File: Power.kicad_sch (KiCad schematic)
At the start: 42 parts, among them J1 1769, U11 XC6206P302MR_C5148691, U6 EA3036C, U7 MT3608, U9 BQ24074RGTR

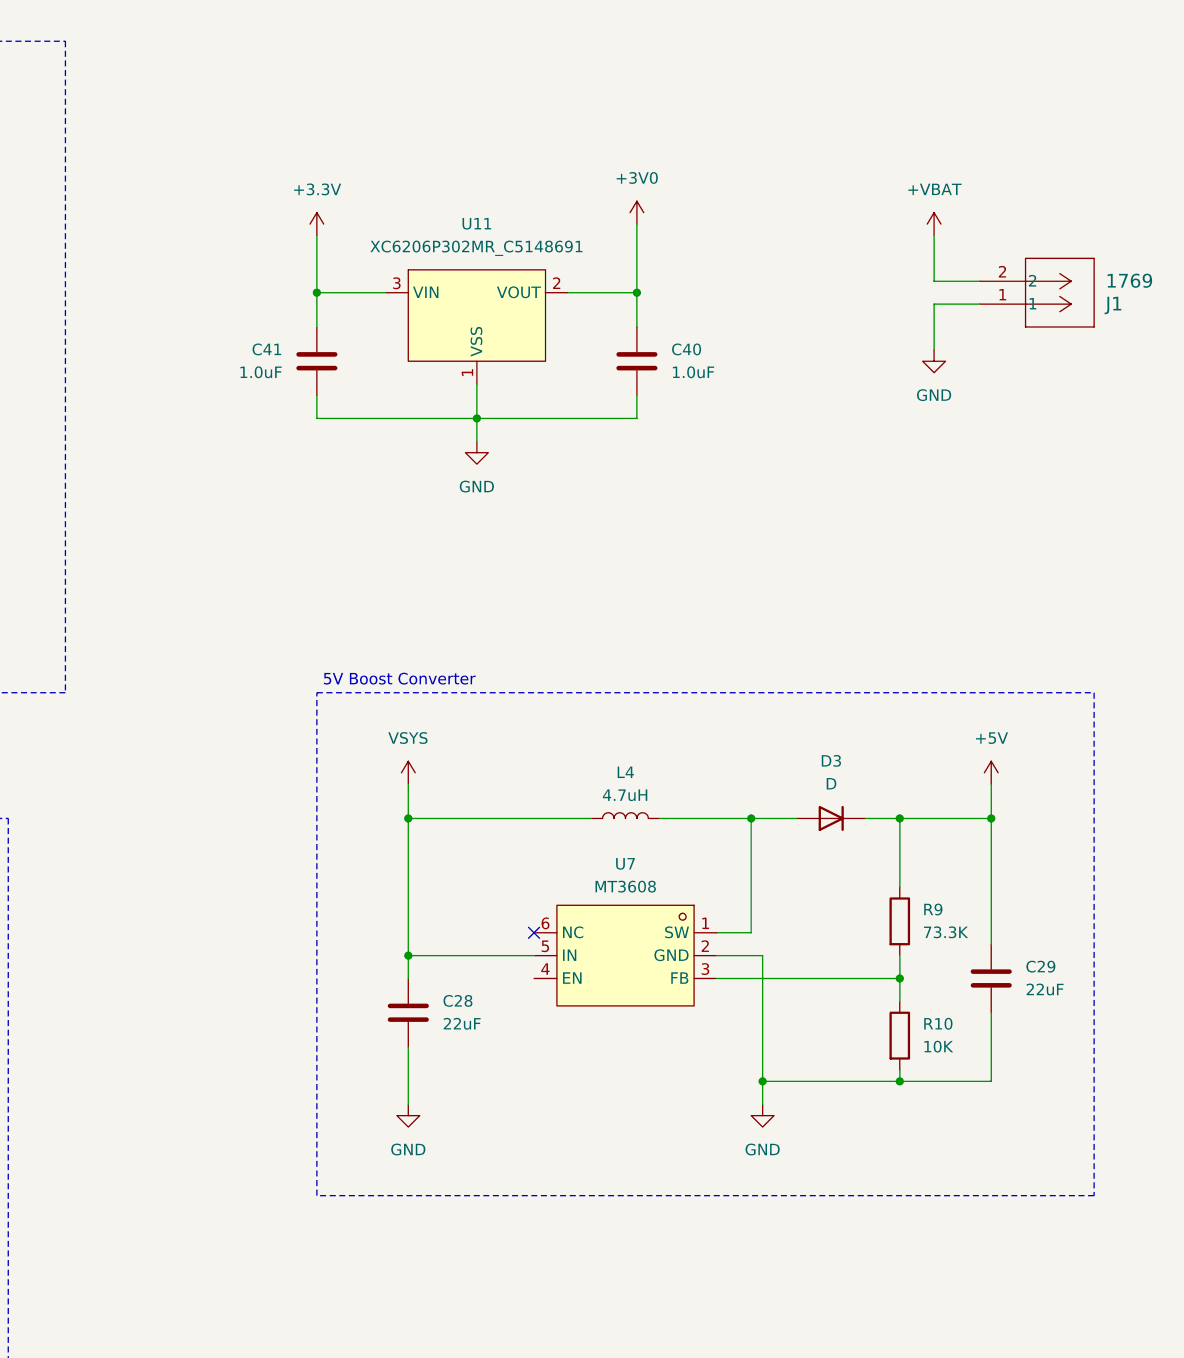
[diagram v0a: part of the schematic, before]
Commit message: power changes for v3s, cleanup
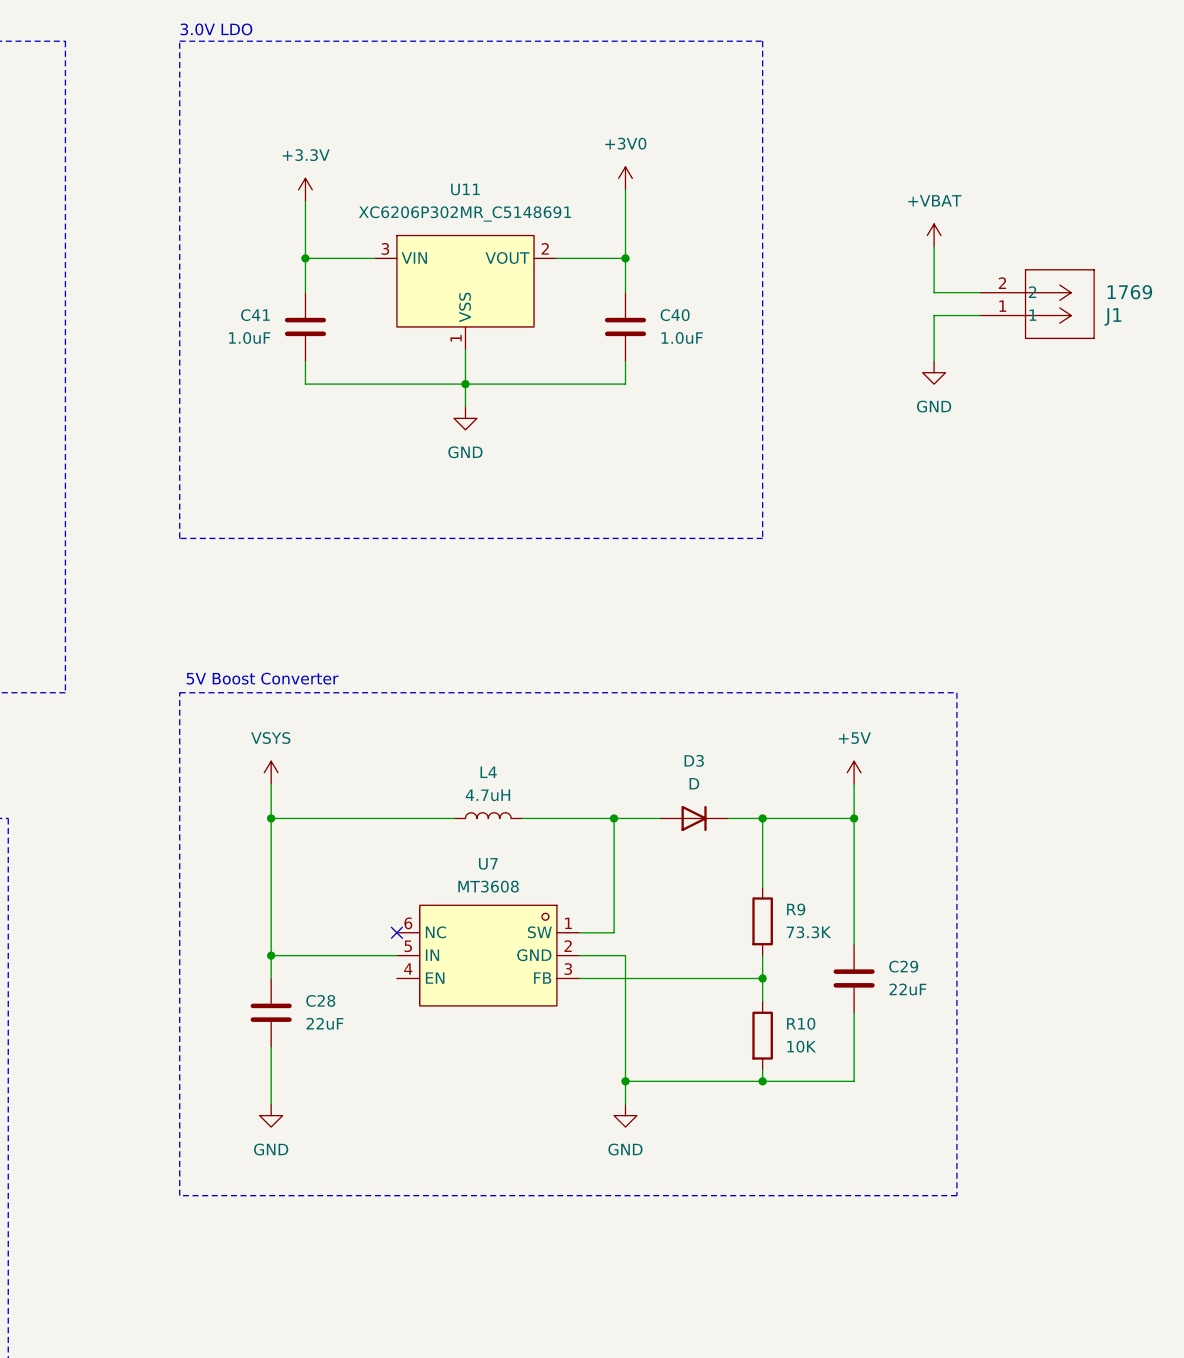
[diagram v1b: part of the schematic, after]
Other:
- note added: "3.0V LDO"
- title: (none) -> iPodClone
- moved on the sheet: C28, C29, C40, C41, D3, J1, L4, R10, R9, U11, U7

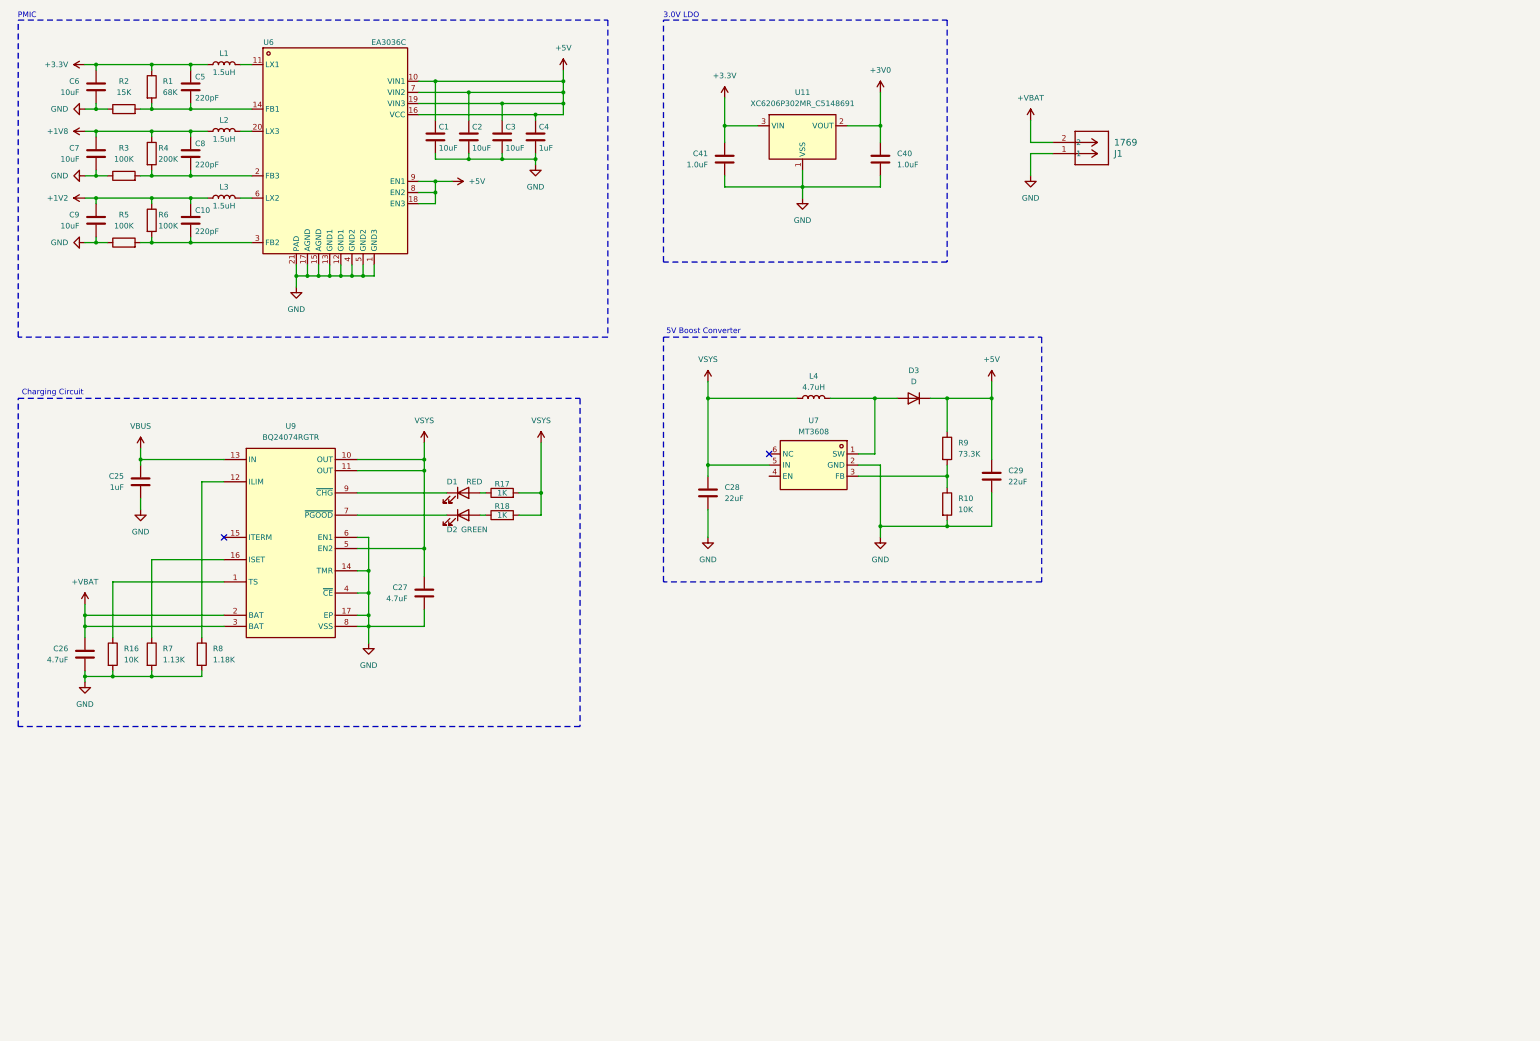
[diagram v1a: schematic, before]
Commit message: gitignore and audio changes
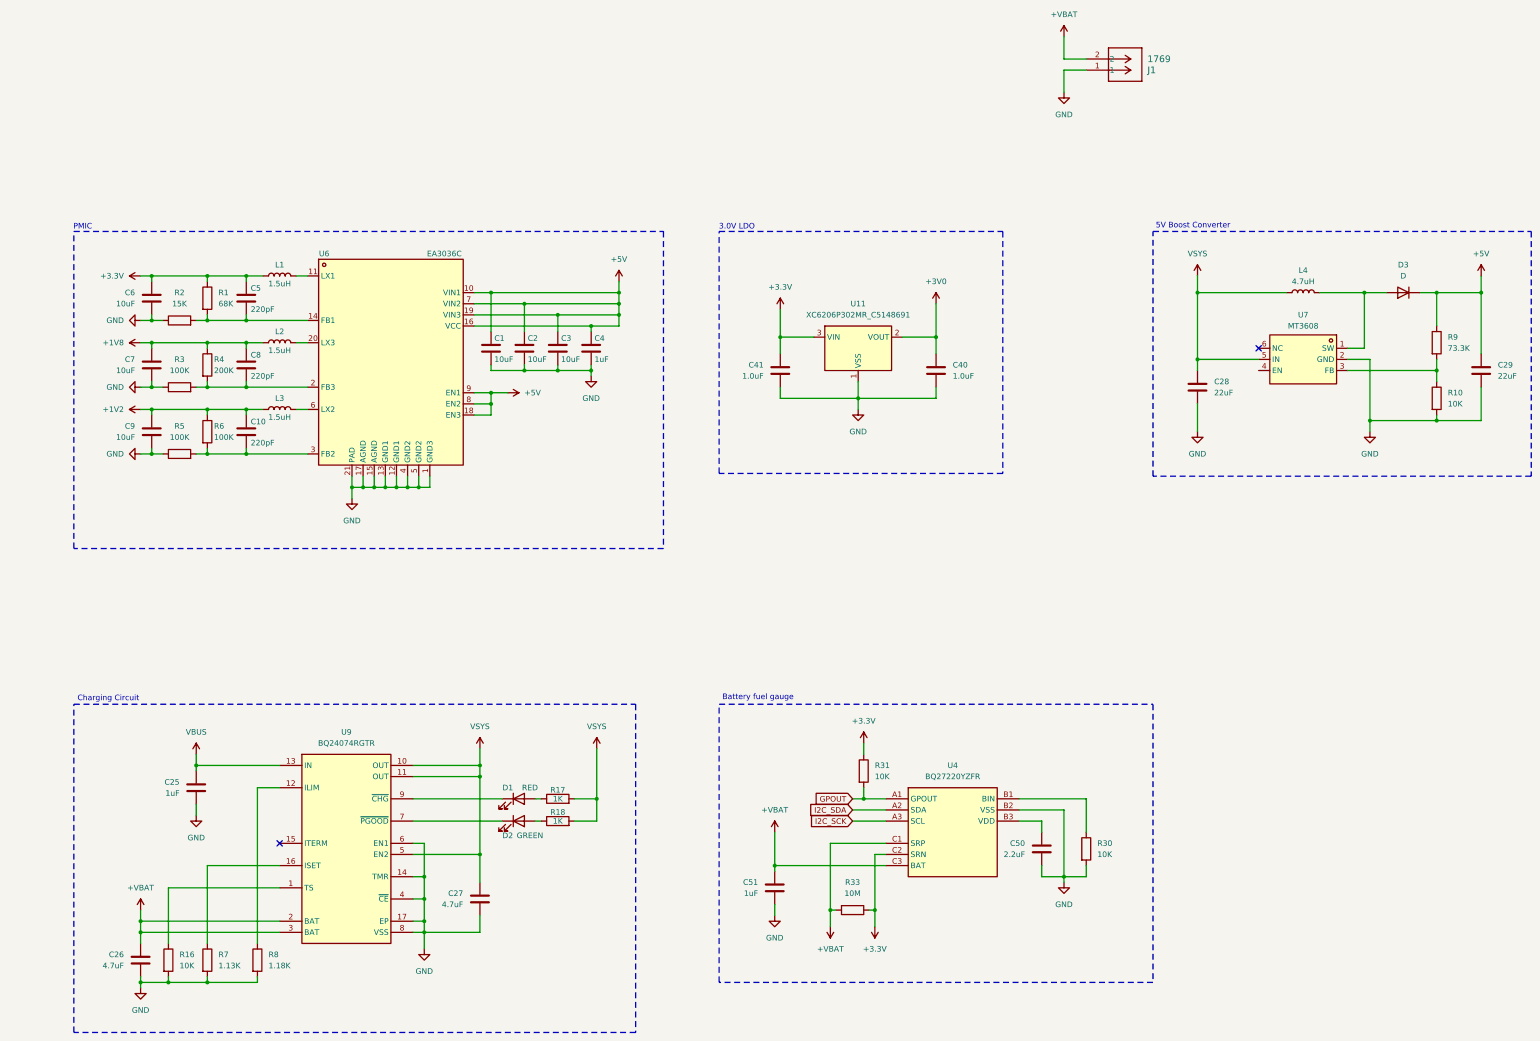
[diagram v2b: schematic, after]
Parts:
- added C50: 2.2uF, symbol Device:C
- added C51: 1uF, symbol Device:C
- added R30, R31: 10K, symbol Device:R
- added R33: 10M, symbol Device:R
- added U4: BQ27220YZFR, easyeda2kicad:DSBGA-9_L1.7-W1.6-R3-C3-P0.50-BL, symbol easyeda2kicad:BQ27220YZFR
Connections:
- net +3.3V: now also R31.1, R33.1, U4.C2 (SRN)
- net +VBAT: now also C51.1, R33.2, U4.C1 (SRP), U4.C3 (BAT)
- net GND: now also C50.2, C51.2, R30.2, U4.B2 (VSS)
- new net: R30.1, U4.B1 (BIN)
- new net: C50.1, U4.B3 (VDD)
- new net GPOUT: R31.2, U4.A1 (GPOUT)
- new net I2C_SCK: U4.A3 (SCL)
- new net I2C_SDA: U4.A2 (SDA)
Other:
- note added: "Battery fuel gauge"
- moved on the sheet: C1, C10, C2, C25, C26, C27, C28, C29, C3, C4, C40, C41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
